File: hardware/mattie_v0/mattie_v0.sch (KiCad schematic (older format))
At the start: 0 parts

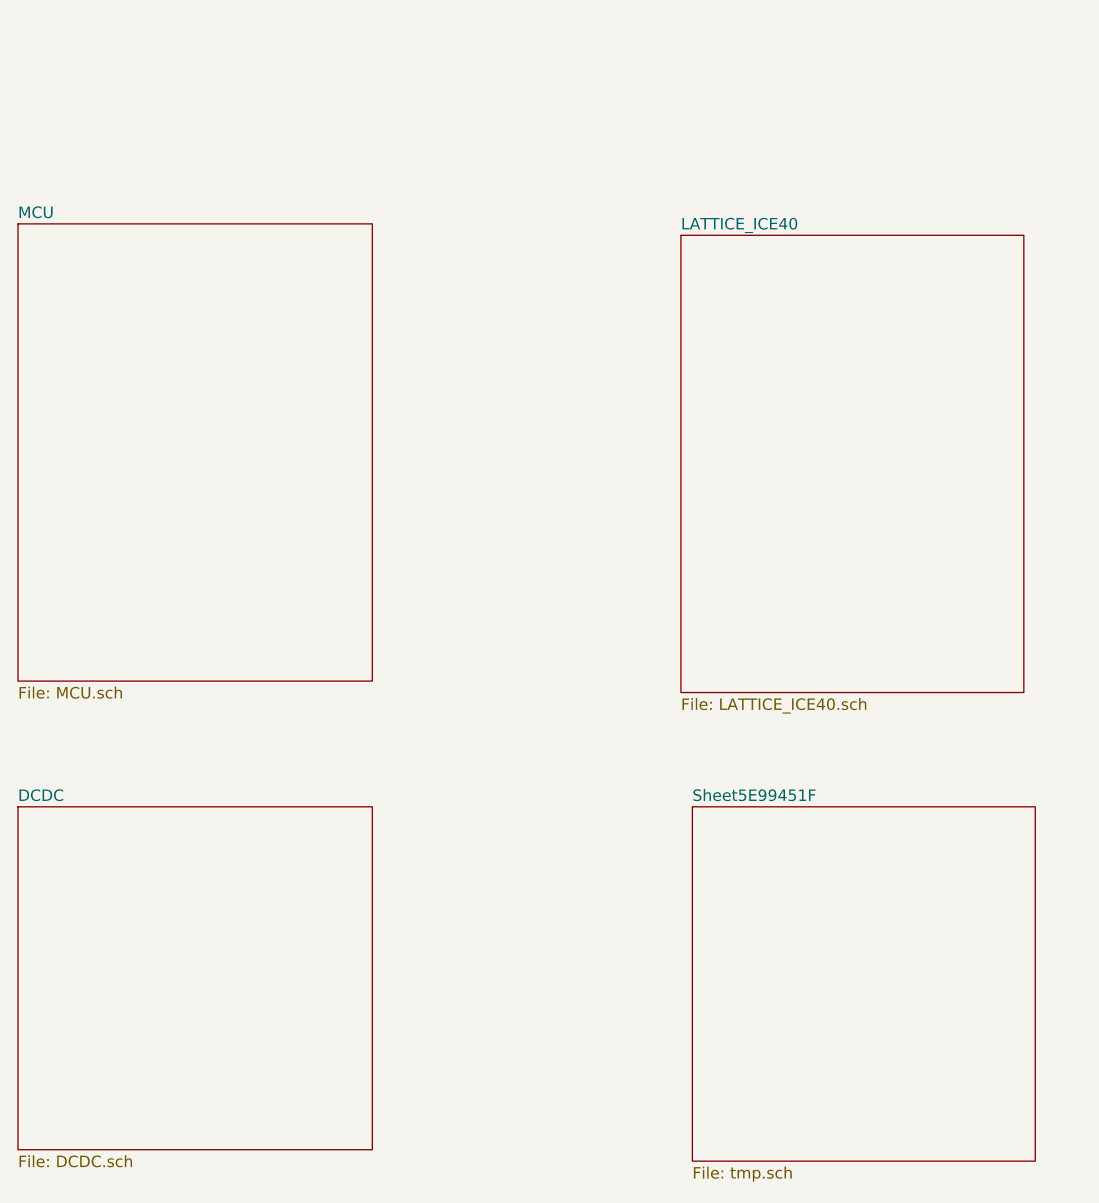
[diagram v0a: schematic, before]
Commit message: update
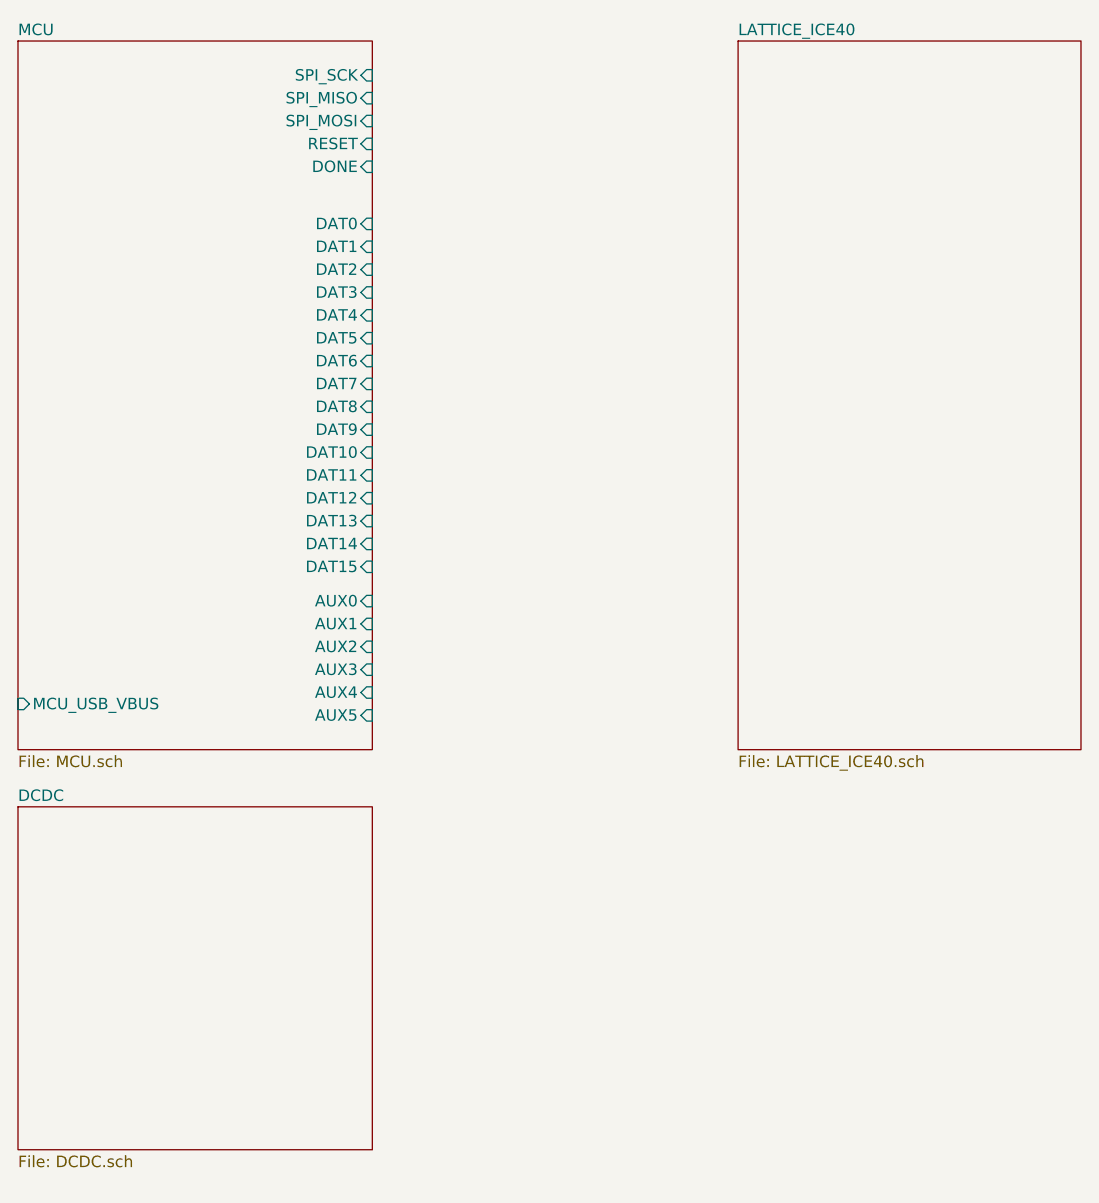
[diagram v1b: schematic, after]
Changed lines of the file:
@@
 $Descr A4 11693 8268
 encoding utf-8
-Sheet 1 5
+Sheet 1 4
 Title "Mattie Version 0"
 Date ""
@@
 $EndDescr
 $Sheet
-S 2400 1800 1550 2000
+S 2400 1000 1550 3100
 U 5E9881B4
 F0 "MCU" 50
 F1 "MCU.sch" 50
+F2 "SPI_SCK" I R 3950 1150 50
+F3 "SPI_MISO" I R 3950 1250 50
+F4 "SPI_MOSI" I R 3950 1350 50
+F5 "RESET" I R 3950 1450 50
+F6 "DONE" I R 3950 1550 50
+F7 "MCU_USB_VBUS" I L 2400 3900 50
+F8 "DAT0" I R 3950 1800 50
+F9 "DAT1" I R 3950 1900 50
+F10 "DAT2" I R 3950 2000 50
+F11 "DAT3" I R 3950 2100 50
+F12 "DAT4" I R 3950 2200 50
+F13 "DAT5" I R 3950 2300 50
+F14 "DAT6" I R 3950 2400 50
+F15 "DAT7" I R 3950 2500 50
+F16 "DAT8" I R 3950 2600 50
+F17 "DAT9" I R 3950 2700 50
+F18 "DAT10" I R 3950 2800 50
+F19 "DAT11" I R 3950 2900 50
+F20 "DAT12" I R 3950 3000 50
+F21 "DAT13" I R 3950 3100 50
+F22 "DAT14" I R 3950 3200 50
+F23 "DAT15" I R 3950 3300 50
+F24 "AUX0" I R 3950 3450 50
+F25 "AUX1" I R 3950 3550 50
+F26 "AUX2" I R 3950 3650 50
+F27 "AUX3" I R 3950 3750 50
+F28 "AUX4" I R 3950 3850 50
+F29 "AUX5" I R 3950 3950 50
 $EndSheet
 $Sheet
@@
 $EndSheet
 $Sheet
-S 5300 1850 1500 2000
+S 5550 1000 1500 3100
 U 5E98823A
 F0 "LATTICE_ICE40" 50
 F1 "LATTICE_ICE40.sch" 50
 $EndSheet
-$Sheet
-S 5350 4350 1500 1550
-U 5E994520
-F0 "Sheet5E99451F" 50
-F1 "tmp.sch" 50
-$EndSheet
 $EndSCHEMATC
